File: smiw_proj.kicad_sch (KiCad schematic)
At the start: 24 parts, among them J1 Conn_02x06_Odd_Even, J2 Conn_02x05_Odd_Even, J3 Conn_01x02, J4 Conn_01x02, SW1 SW_Push, U1 LM2596S-5, U2 M5 Stamp-S3, U3 LD1117S33TR_SOT223

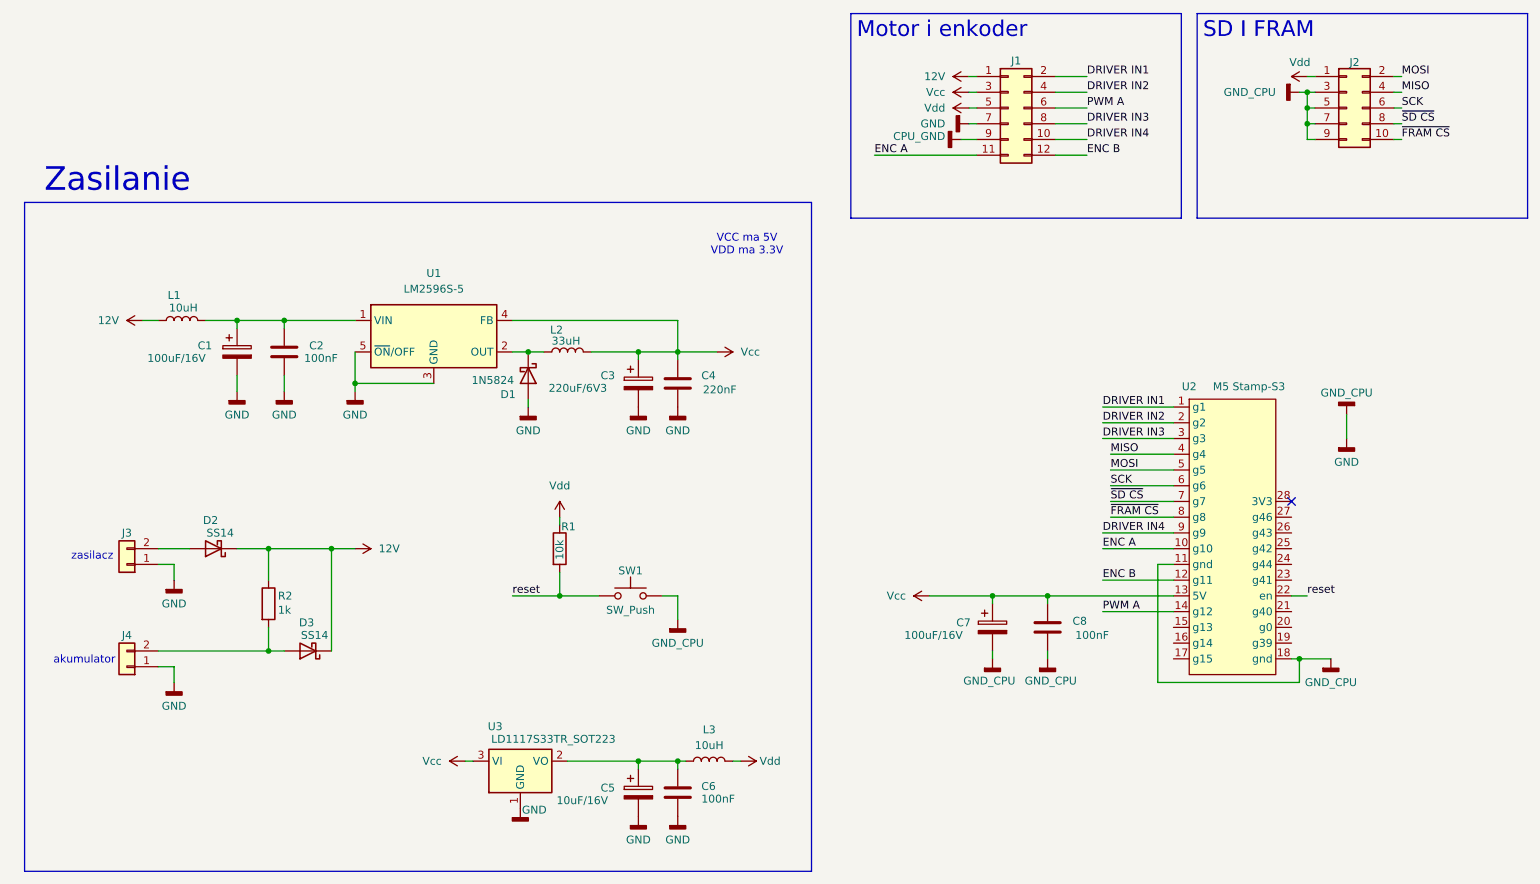
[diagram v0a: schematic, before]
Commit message: pcb dobrze zdaniem michala (to nie ma sensu)
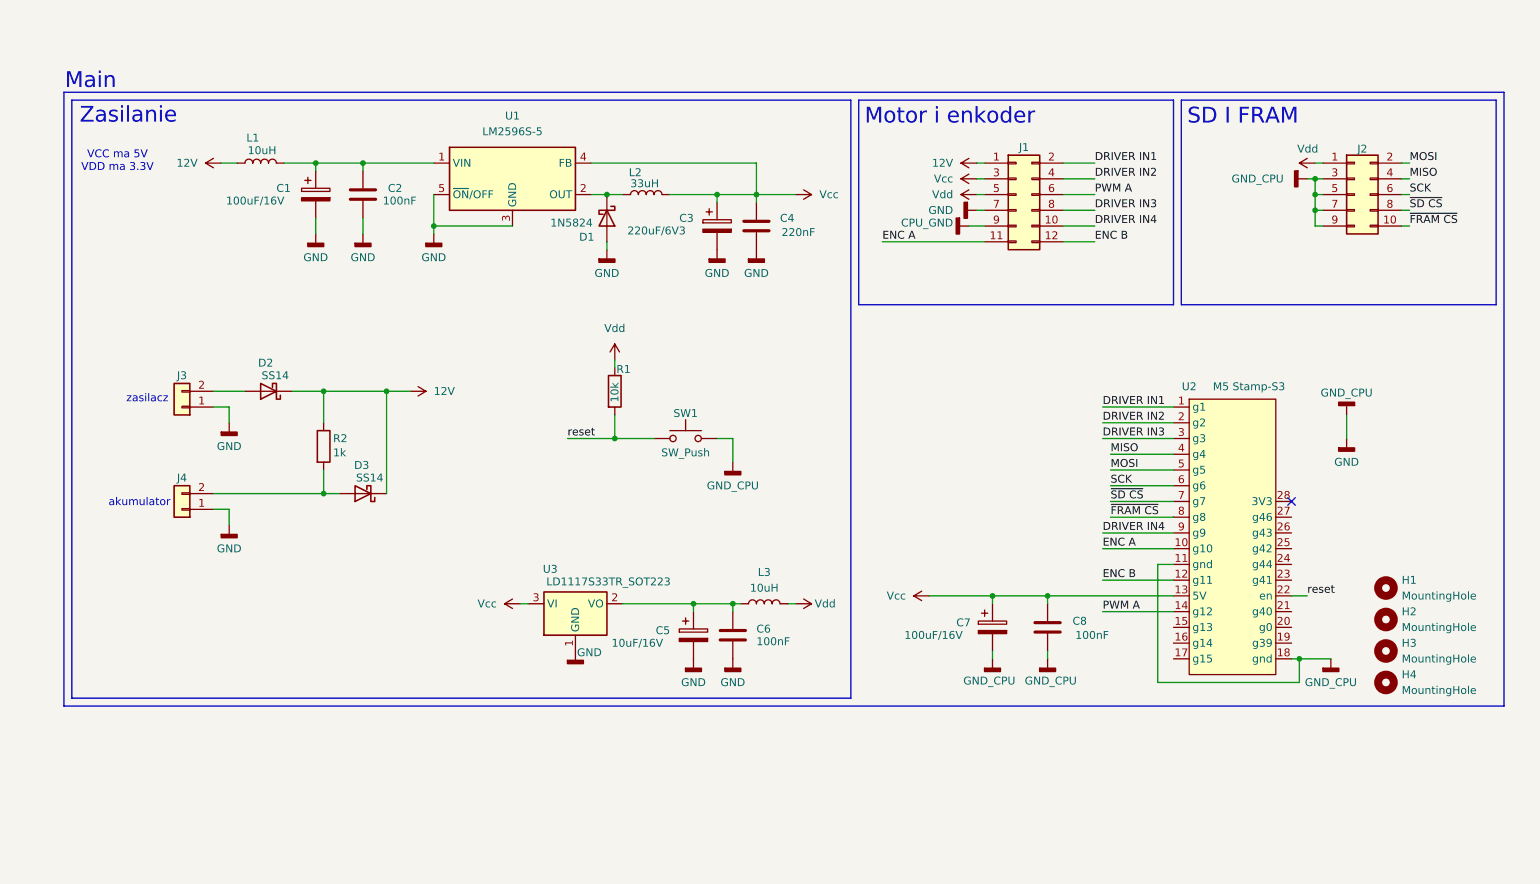
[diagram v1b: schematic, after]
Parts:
- added H1, H2, H3, H4: MountingHole, MountingHole:MountingHole_3.2mm_M3_DIN965_Pad_TopBottom, symbol Mechanical:MountingHole
- J1: footprint Connector_PinSocket_1.00mm:PinSocket_2x05_P1.00mm_Vertical_SMD -> Connector_PinHeader_2.54mm:PinHeader_2x06_P2.54mm_Vertical
- J2: footprint Connector_PinSocket_1.00mm:PinSocket_2x05_P1.00mm_Vertical_SMD -> Connector_PinSocket_2.54mm:PinSocket_2x05_P2.54mm_Vertical_SMD
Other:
- note added: "Main"
- moved on the sheet: C1, C2, C3, C4, C5, C6, D1, D2, D3, J1, J2, J3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
